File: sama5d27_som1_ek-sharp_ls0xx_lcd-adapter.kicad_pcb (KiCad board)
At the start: 2 copper layers, 50.1 x 80.2 mm, 14 parts, among them J1 XF2M-5015-1A, J2 51441-1093

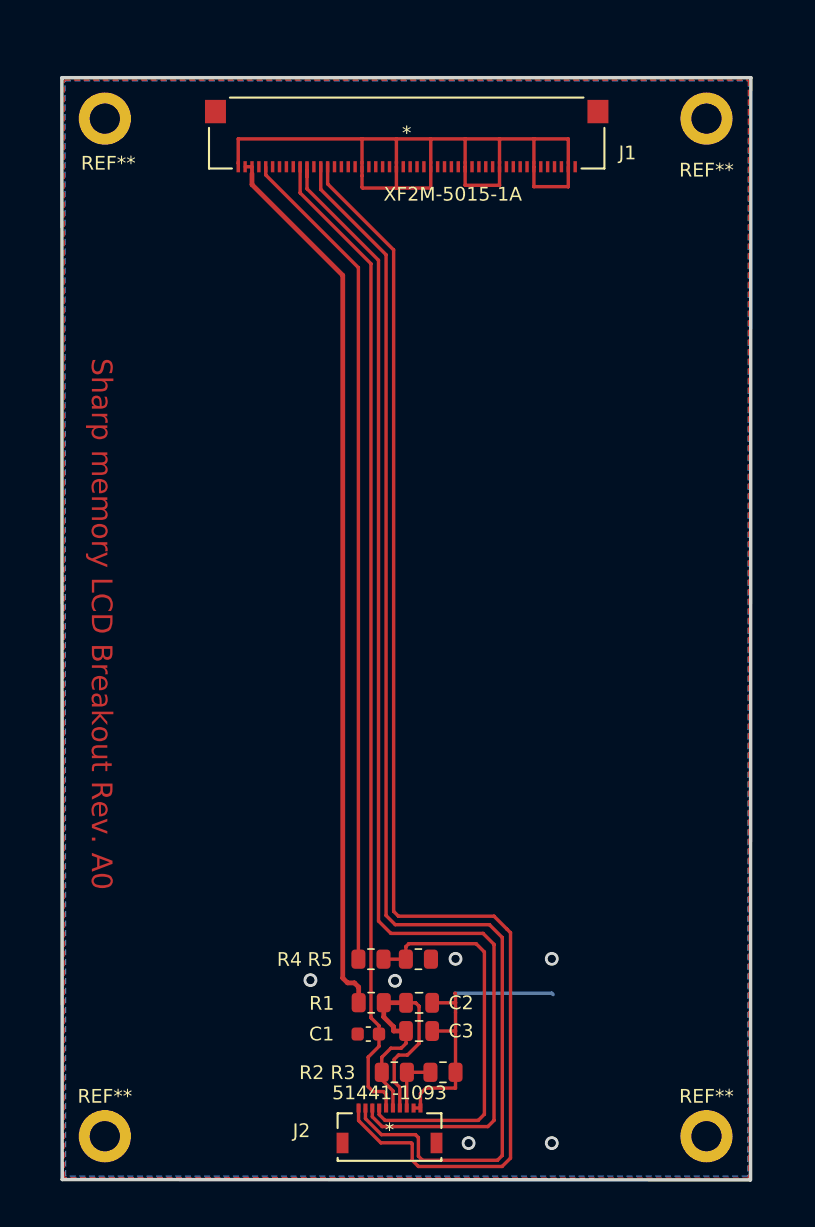
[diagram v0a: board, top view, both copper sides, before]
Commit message: Update RevA1
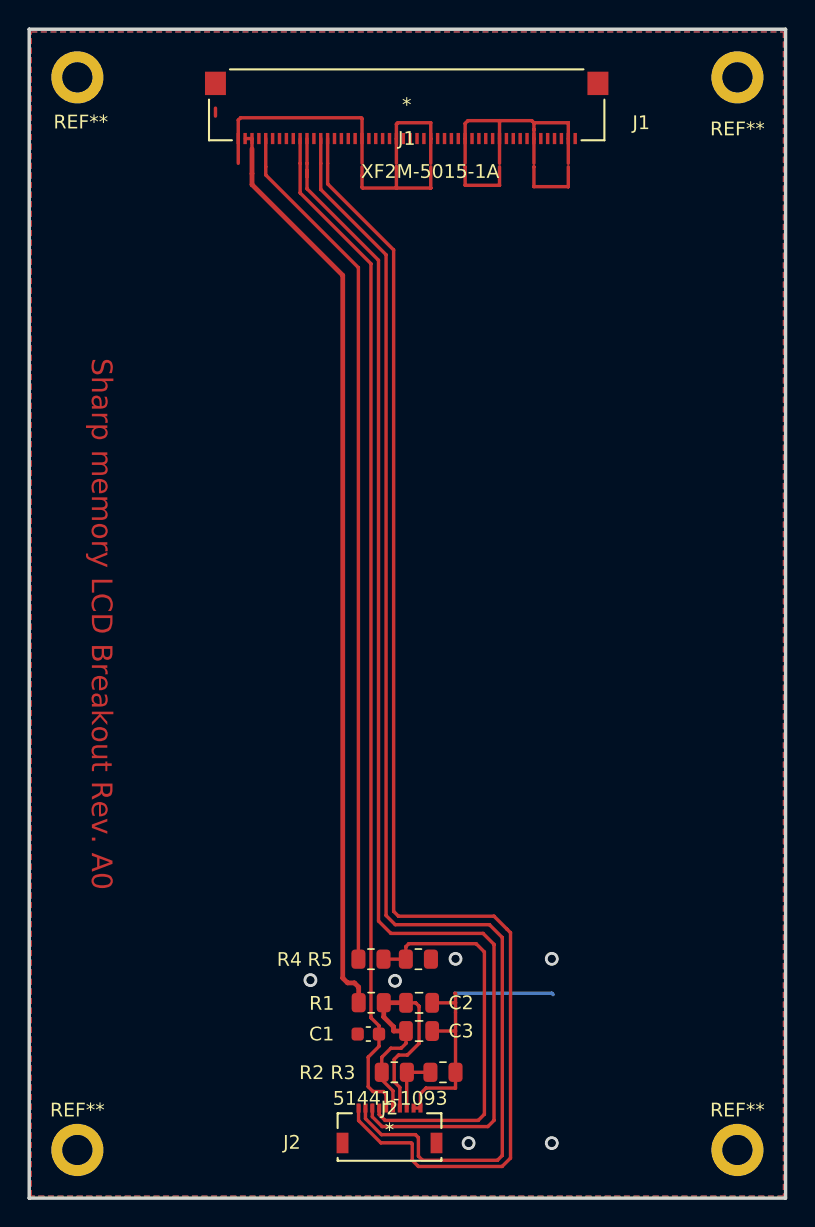
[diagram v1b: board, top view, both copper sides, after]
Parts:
- moved REF** 3.75 mm to (211.5, 22.5)
- moved REF** 3.61 mm to (163.5, 22.5)
- moved REF** 2.46 mm to (211.5, 100.5)
- moved REF** 2.24 mm to (163.5, 100.5)
- moved J1 2.05 mm to (187.4, 24.5)
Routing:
- net GND: track 80.9 -> 85.9 mm
- net /LCD_PWM: track 60.4 -> 62.5 mm
- net /5V: track 64.8 -> 66.8 mm
- net /SPI0_SPCK_SCK: track 96.4 -> 98.2 mm
- net /SPI0_NPCS0_SCS: track 89.8 -> 91.6 mm
- net /SPI0_MOSI_SI: track 94.5 -> 96.3 mm
- net /LCD_DISP_DISP: track 72.4 -> 74.2 mm
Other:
- board size 50.1 x 80.2 mm -> 55 x 85 mm
- board text added: "J1"
- board text added: "J2"

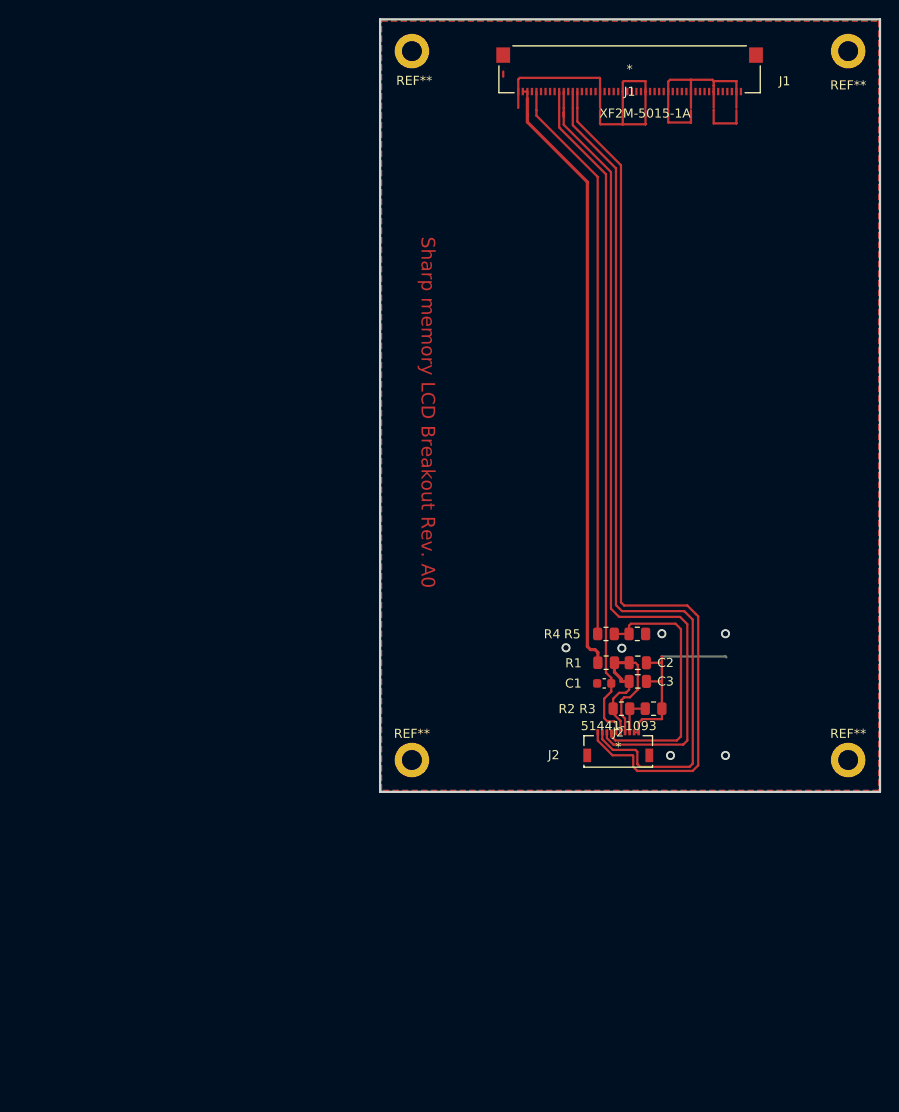
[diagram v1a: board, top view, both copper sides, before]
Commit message: Centralize pcb in sheet
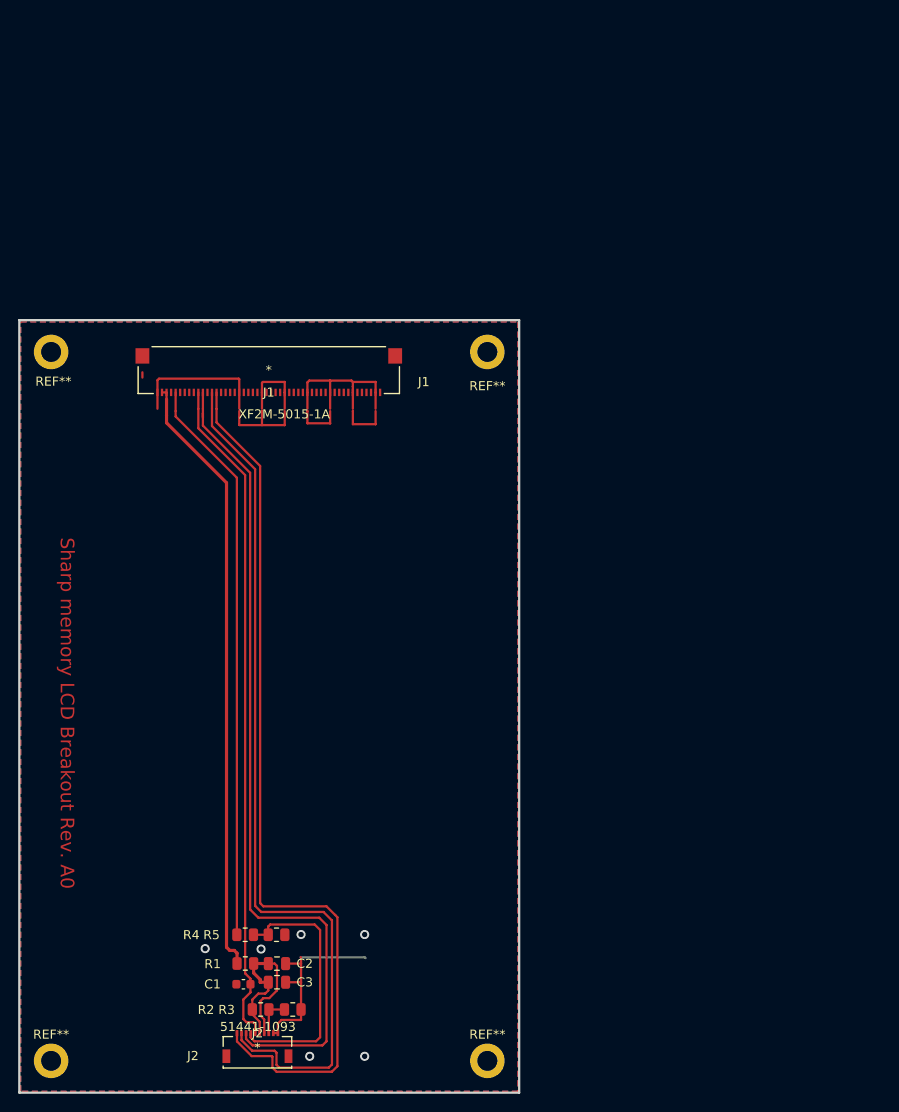
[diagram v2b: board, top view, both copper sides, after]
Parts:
- moved R2 51.7 mm to (146.8, 128.0)
- moved R3 51.7 mm to (150.4, 128.0)
- moved R1 51.7 mm to (145.2, 122.9)
- moved R5 51.7 mm to (148.6, 119.7)
- moved REF** 51.7 mm to (123.8, 55.6)
- moved REF** 51.7 mm to (123.8, 133.6)
- moved C1 51.7 mm to (145.0, 125.2)
- moved C2 51.7 mm to (148.7, 122.9)
- moved C3 51.7 mm to (148.7, 125.0)
- moved J1 51.7 mm to (147.7, 57.6)
- moved J2 51.7 mm to (146.5, 132.2)
- moved REF** 51.7 mm to (171.8, 55.6)
- moved R4 51.7 mm to (145.2, 119.7)
- moved REF** 51.7 mm to (171.8, 133.6)
